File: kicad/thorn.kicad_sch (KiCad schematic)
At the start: 26 parts, among them J3 Conn_01x09, SW11 SW_Push, SW12 SW_Push, U1 RP2040, U3 W25Q128JVS, Y1 Crystal_GND24

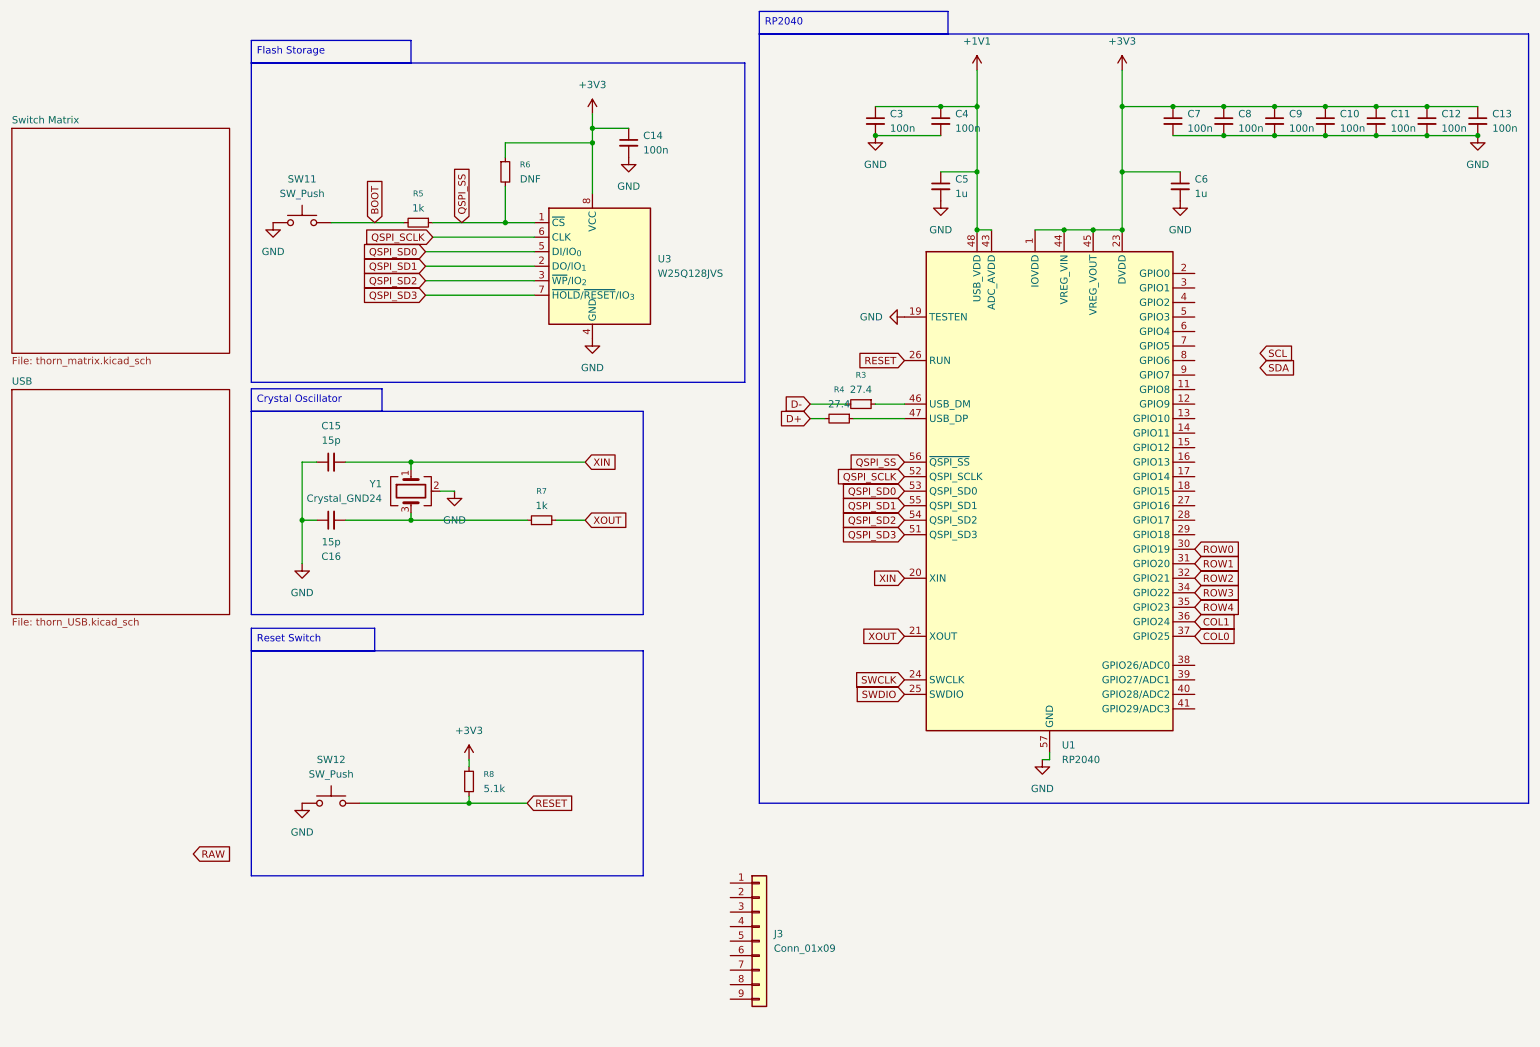
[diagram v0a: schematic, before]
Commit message: feat: finished preliminary wiring
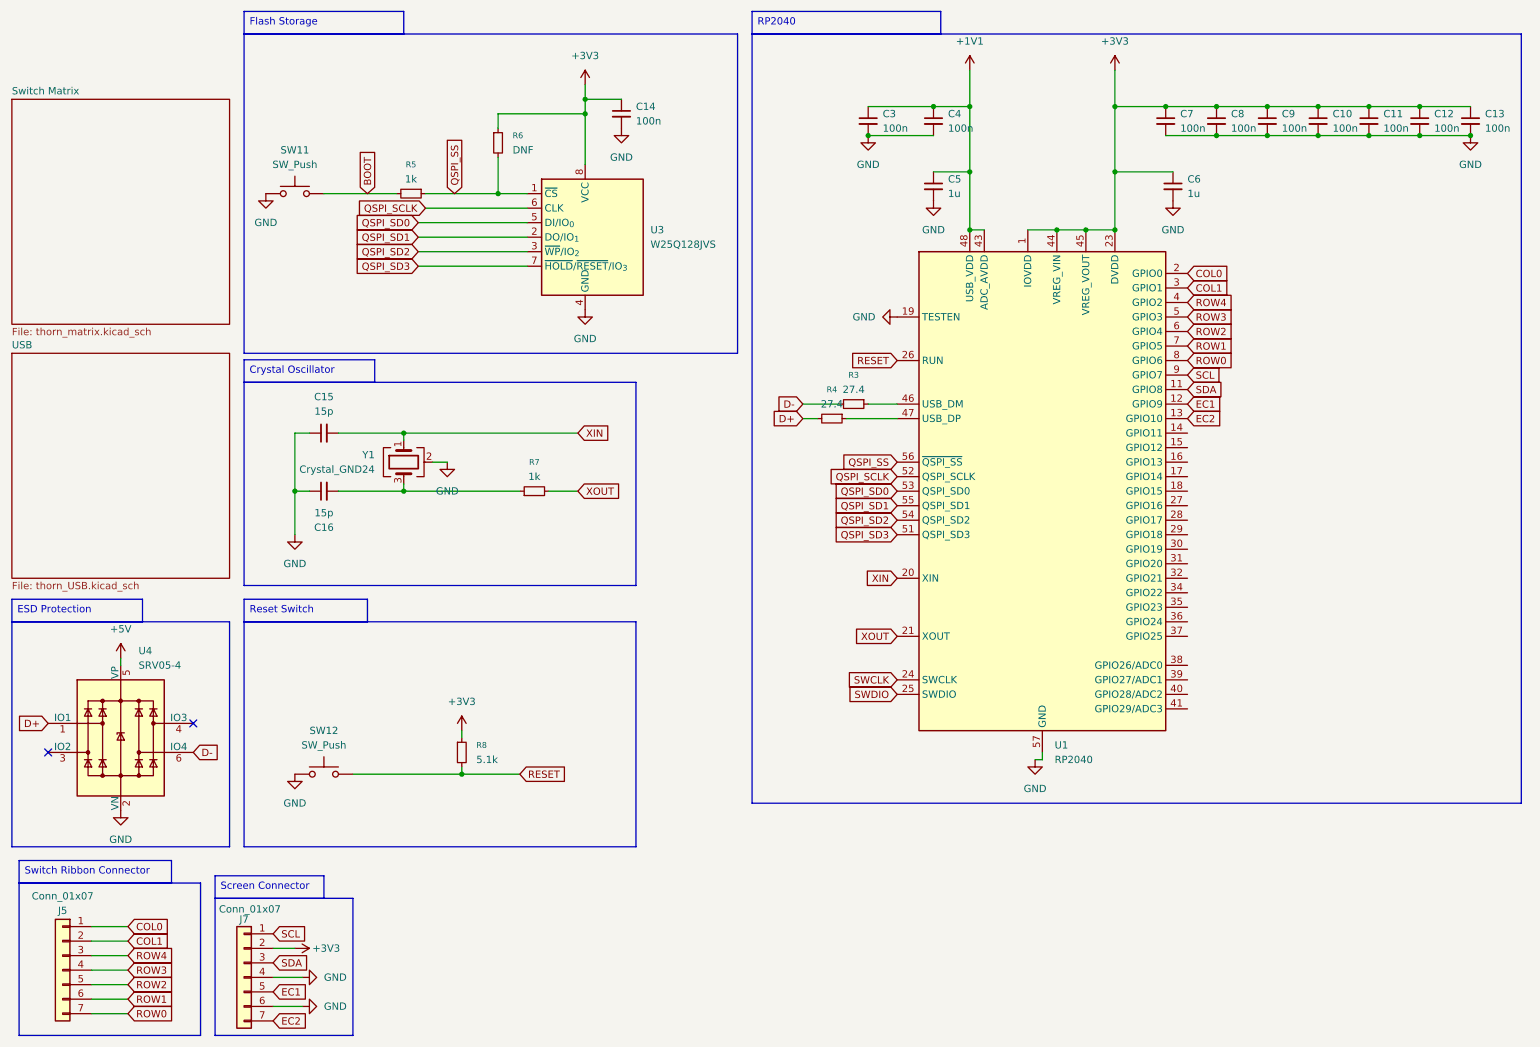
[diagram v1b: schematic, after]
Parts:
- removed J3: Conn_01x09, symbol Connector_Generic:Conn_01x09
- added J5, J7: Conn_01x07, Connector_FFC-FPC:Molex_200528-0070_1x07-1MP_P1.00mm_Horizontal, symbol Connector_Generic:Conn_01x07
- added U4: SRV05-4, Package_TO_SOT_SMD:SOT-23-6, symbol Power_Protection:SRV05-4
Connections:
- net +3V3: now also J7.2 (Pin_2)
- net COL0: now also U1.2 (GPIO0), J5.1 (Pin_1); no longer U1.37 (GPIO25)
- net COL1: now also U1.3 (GPIO1), J5.2 (Pin_2); no longer U1.36 (GPIO24)
- net D+: now also U4.1 (IO1)
- net D-: now also U4.6 (IO4)
- net GND: now also J7.4 (Pin_4), J7.6 (Pin_6), U4.2 (VN)
- net ROW0: now also U1.8 (GPIO6), J5.7 (Pin_7); no longer U1.30 (GPIO19)
- net ROW1: now also U1.7 (GPIO5), J5.6 (Pin_6); no longer U1.31 (GPIO20)
- net ROW2: now also U1.6 (GPIO4), J5.5 (Pin_5); no longer U1.32 (GPIO21)
- net ROW3: now also U1.5 (GPIO3), J5.4 (Pin_4); no longer U1.34 (GPIO22)
- net ROW4: now also U1.4 (GPIO2), J5.3 (Pin_3); no longer U1.35 (GPIO23)
- net SCL: now also U1.9 (GPIO7), J7.1 (Pin_1)
- net SDA: now also U1.11 (GPIO8), J7.3 (Pin_3)
- net EC1: now reaches U1.12 (GPIO9)
- net EC1: now also J7.5 (Pin_5)
- net EC2: now reaches U1.13 (GPIO10)
- net EC2: now also J7.7 (Pin_7)
- new net +5V: U4.5 (VP)
- no-connect marks 0 -> 2
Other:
- moved on the sheet: C10, C11, C12, C13, C14, C15, C16, C3, C4, C5, C6, C7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

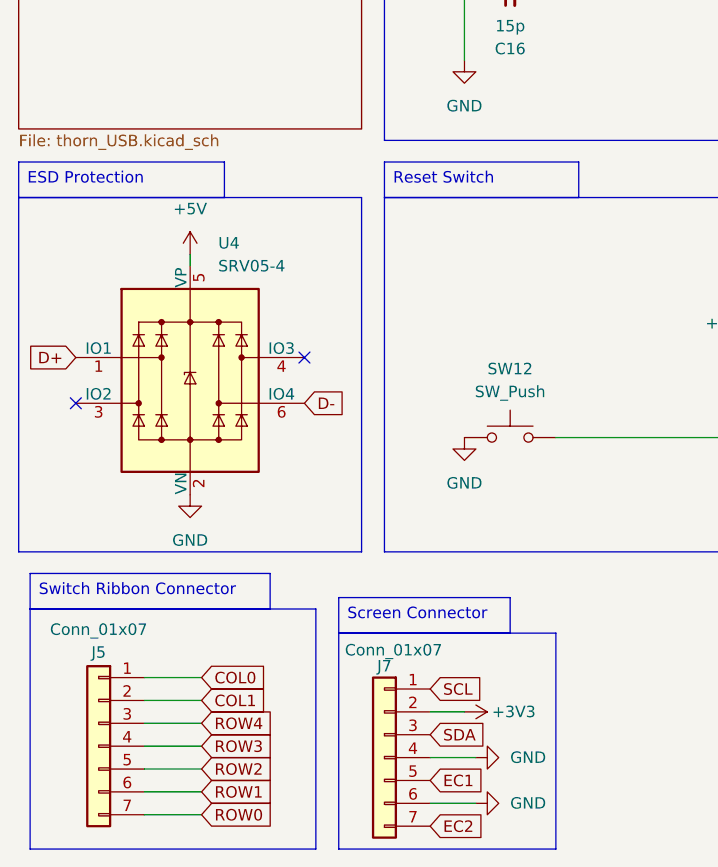
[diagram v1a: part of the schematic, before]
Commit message: feat: change pcb to preliminary final design
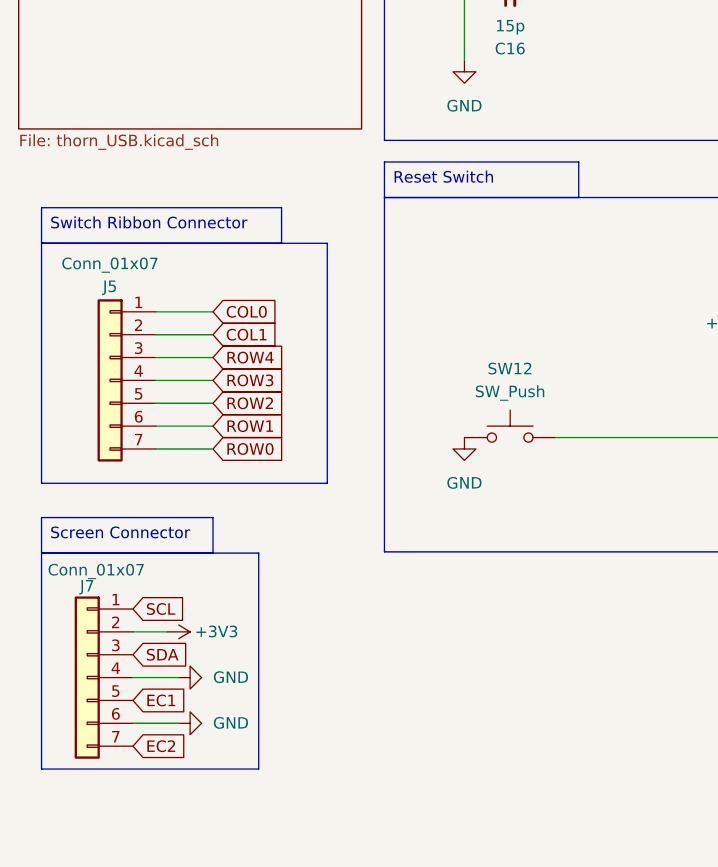
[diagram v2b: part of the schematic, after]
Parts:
- removed U4: SRV05-4, Package_TO_SOT_SMD:SOT-23-6, symbol Power_Protection:SRV05-4
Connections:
- no-connect marks 2 -> 0
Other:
- moved on the sheet: J5, J7
